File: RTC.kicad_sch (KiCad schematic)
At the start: 12 parts, among them J7 Molex 470531000, U1 PCF8563T, U10 EMC2301-1-ACZL-TR, U11 74LVC1G07SE-7, Y2 X32K768S301

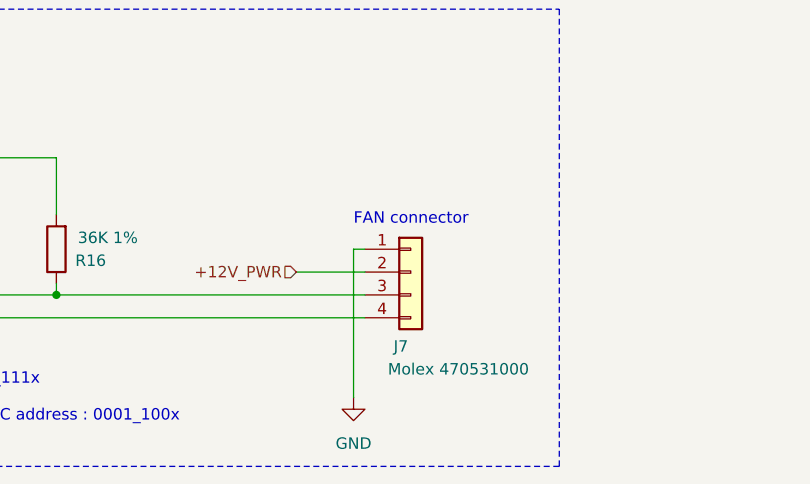
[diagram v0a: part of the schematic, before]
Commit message: we ballin??
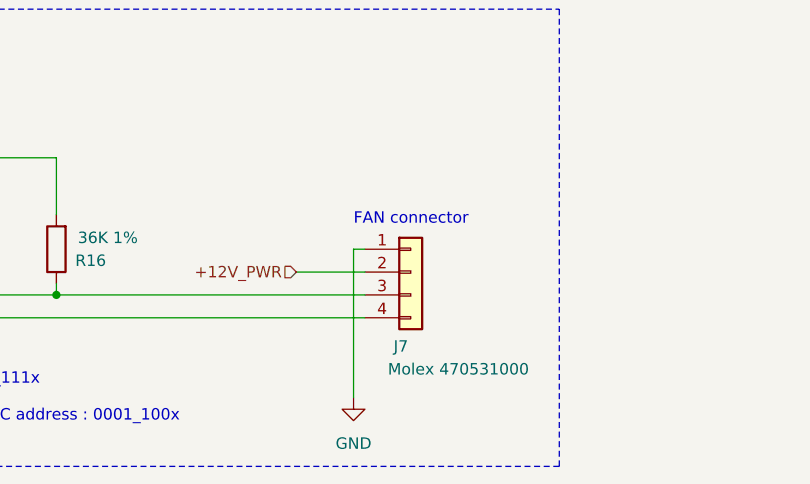
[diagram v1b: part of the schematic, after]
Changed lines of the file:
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@@
 			)
 		)
-		(property "Description" ""
+		(property "Description" "Two pin crystal, small symbol"
 			(at 58.42 53.34 0)
 			(effects
@@
 			)
 		)
-		(property "Datasheet" "https://ww1.microchip.com/downloads/en/DeviceDoc/2301.pdf"
+		(property "Datasheet" "https://ww1.microchip.com/downloads/aemDocuments/documents/MSLD/ProductDocuments/DataSheets/EMC2301-2-3-5-Data-Sheet-DS20006532A.pdf"
 			(at 121.92 139.7 0)
 			(effects
@@
 			)
 		)
-		(property "Datasheet" "https://www.molex.com/pdm_docs/sd/470531000_sd.pdf"
+		(property "Datasheet" "~"
 			(at 176.53 132.08 0)
 			(effects
@@
 			)
 		)
-		(property "Description" ""
+		(property "Description" "Generic connector, single row, 01x04, script generated (kicad-library-utils/schlib/autogen/connector/)"
 			(at 176.53 132.08 0)
 			(effects
